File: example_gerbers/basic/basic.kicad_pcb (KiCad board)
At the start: 2 copper layers, 10 x 15 mm, 0 parts

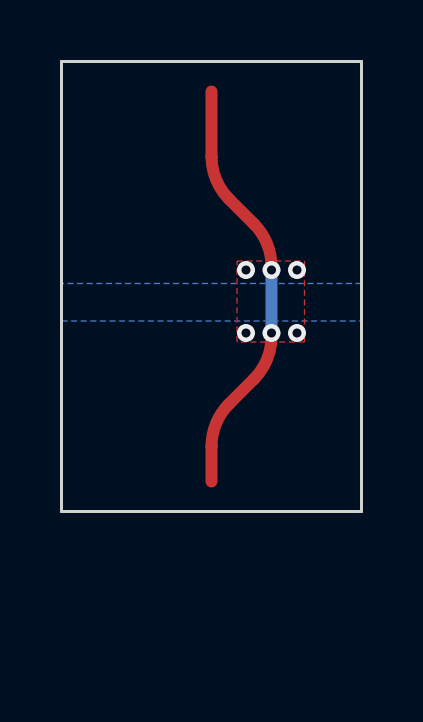
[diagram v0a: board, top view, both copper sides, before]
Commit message: Updated basic example
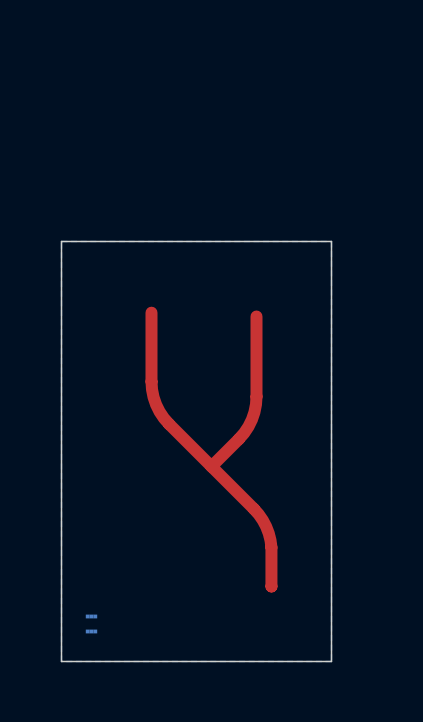
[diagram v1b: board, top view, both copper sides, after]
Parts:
- added SP1: Simulation-Port, antmicro-footprints:Simulation-Port, F.Cu at (143.0, 103.3)
- added SP2: Simulation-Port, antmicro-footprints:Simulation-Port, F.Cu at (147.0, 112.6)
- added TP1: Net-Tie_2, antmicro-footprints:NetTie-2_SMD_Pad0.127mm, F.Cu at (143.0, 103.5)
- added TP2: Net-Tie_2, antmicro-footprints:NetTie-2_SMD_Pad0.127mm, B.Cu at (141.0, 114.0)
- added TP3: Net-Tie_2, antmicro-footprints:NetTie-2_SMD_Pad0.127mm, F.Cu at (147.0, 112.4)
- added TP4: Net-Tie_2, antmicro-footprints:NetTie-2_SMD_Pad0.127mm, B.Cu at (141.0, 113.5)
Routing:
- net /MSL: track 0.00 -> 16.1 mm
- net /A: track 14.3 -> 0.00 mm, vias 2 -> 0
- net /B: vias 4 -> 0
- added copper zone on B.Cu, net GND
- removed copper zone on B.Cu, net /B
- removed copper zone on F.Cu, net /B
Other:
- board size 10 x 15 mm -> 9 x 14 mm
